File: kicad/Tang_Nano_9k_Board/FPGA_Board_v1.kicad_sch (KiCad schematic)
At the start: 51 parts, among them J1 Conn_01x24, J2 Conn_01x24, J3 Conn_01x08, J4 Conn_01x04, J5 Conn_01x04, J6 Conn_01x04, J7 Conn_01x04, Q1 PMOS, Q2 PMOS, Q3 PMOS, Q4 PMOS, Q5 PMOS, Q6 PMOS, Q7 PMOS, Q8 PMOS, SW1 SW_DIP_x08, SW2 SW_Push, SW3 SW_Push, SW4 SW_Push, U3 TBD62083AFG, U4 74HC138

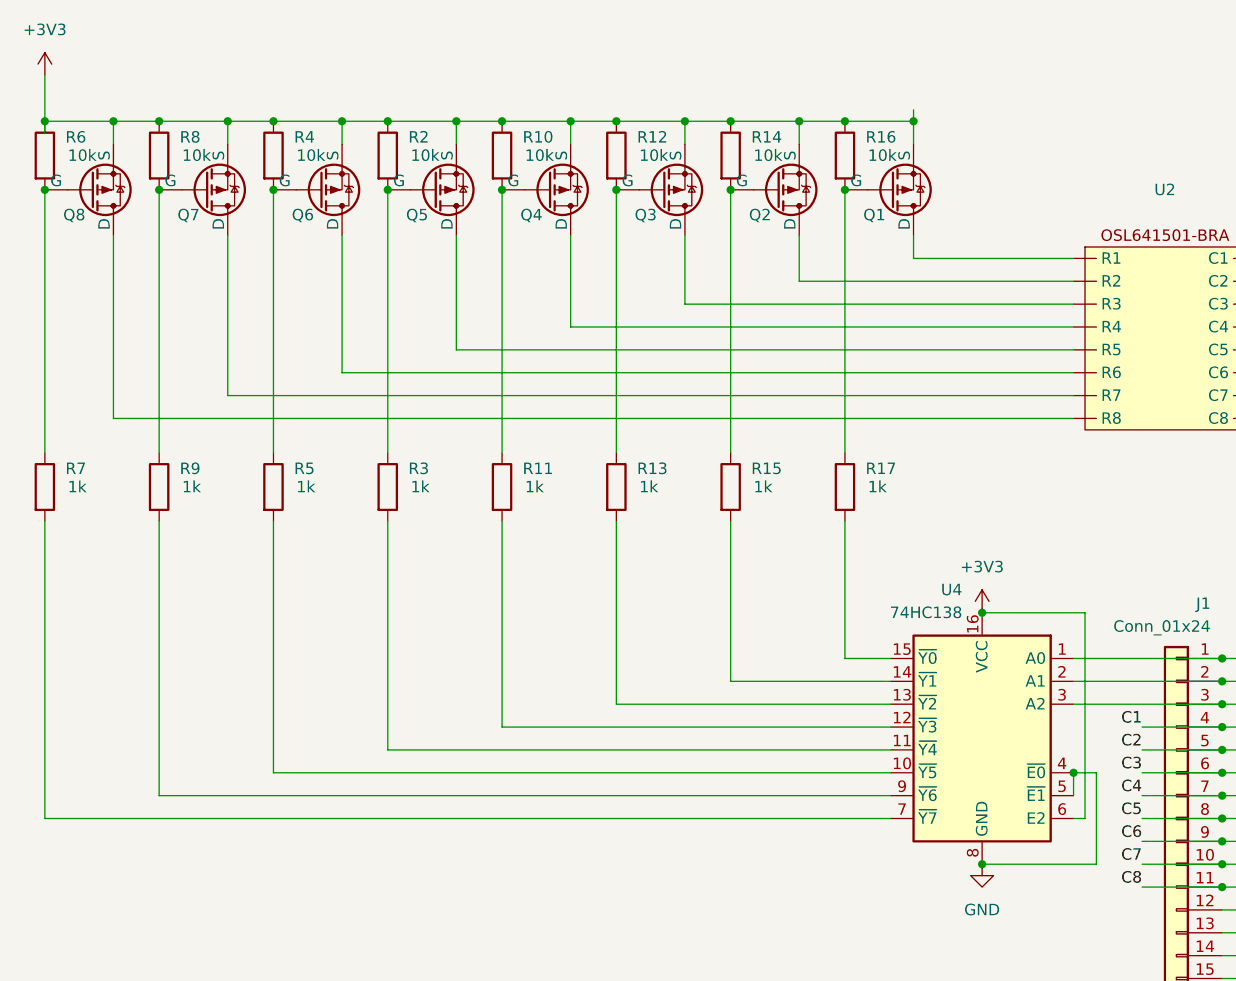
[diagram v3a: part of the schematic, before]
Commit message: set footprint
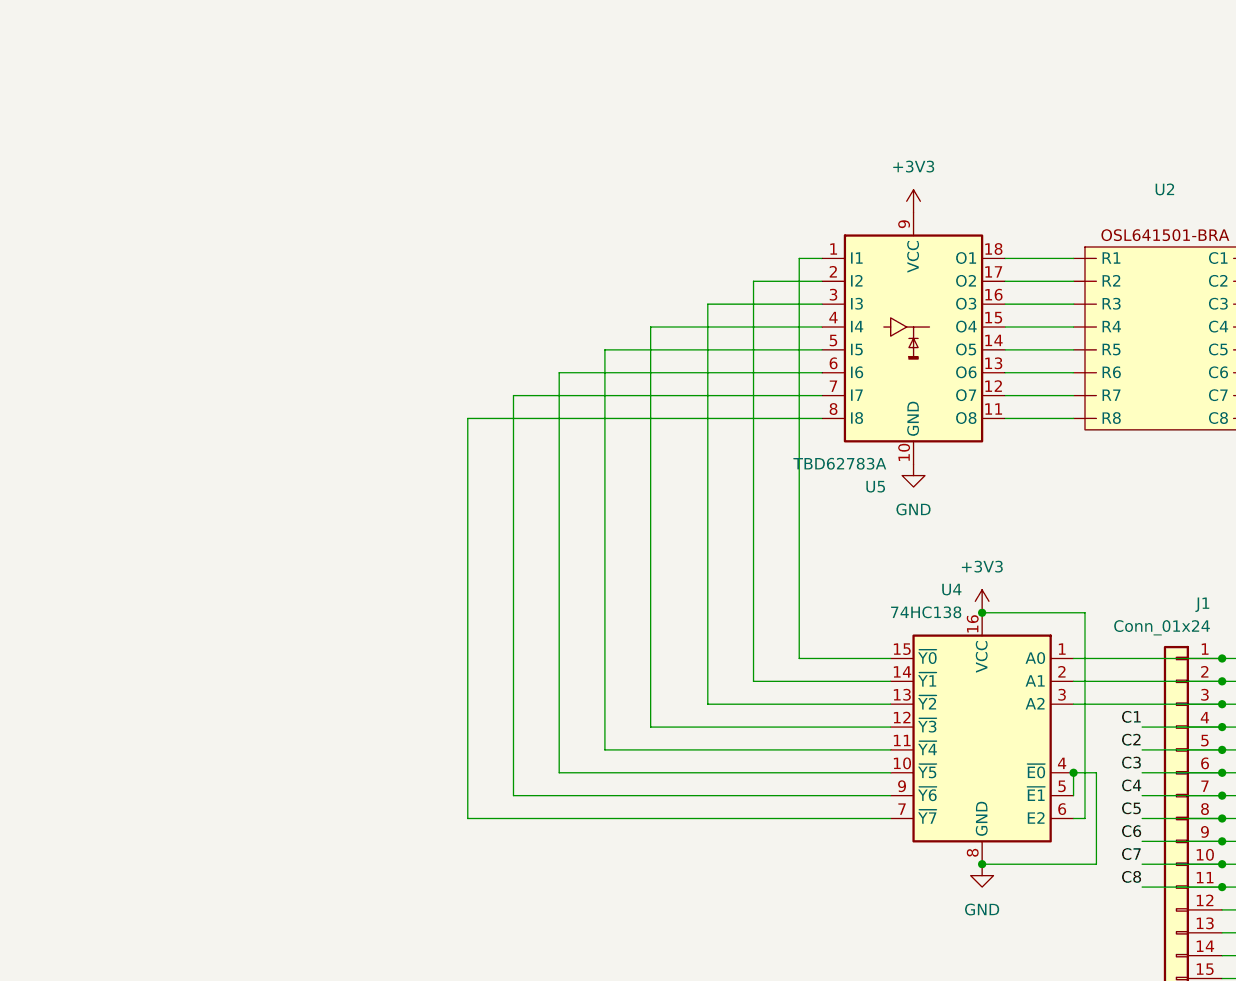
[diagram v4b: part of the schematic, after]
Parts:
- removed Q1, Q2, Q3, Q4, Q5, Q6, Q7, Q8: PMOS, symbol Simulation_SPICE:PMOS
- removed R10, R12, R14, R16, R2, R4, R6, R8: 10k, symbol Device:R
- removed R11, R13, R15, R17, R3, R5, R7, R9: 1k, symbol Device:R
- added U5: TBD62783A, Package_DIP:DIP-18_W7.62mm, symbol Transistor_Array:TBD62783A
- H1, H2, H3, H4: footprint (none) -> MountingHole:MountingHole_2.1mm
- J1, J2: footprint (none) -> Connector_PinHeader_2.54mm:PinHeader_1x24_P2.54mm_Vertical
- J3: footprint (none) -> Connector_PinHeader_2.54mm:PinHeader_1x08_P2.54mm_Vertical
- J4, J5, J6, J7: footprint (none) -> Connector_PinHeader_2.54mm:PinHeader_1x04_P2.54mm_Vertical
- R18, R19, R20, R21, R22, R23, R24, R25: footprint (none) -> Resistor_THT:R_Axial_DIN0207_L6.3mm_D2.5mm_P7.62mm_Horizontal
- SW1: footprint (none) -> Button_Switch_THT:SW_DIP_SPSTx07_Slide_9.78x19.96mm_W7.62mm_P2.54mm
- SW2, SW3, SW4: footprint (none) -> Button_Switch_SMD:Panasonic_EVQPUJ_EVQPUA
- U1: footprint (none) -> BFP:Tang_Nano_9K
- U2: footprint (none) -> BFP:OSL641501-BX
- U4: footprint (none) -> Package_DIP:CERDIP-16_W7.62mm_SideBrazed
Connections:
- net +3V3: now also U5.9 (VCC)
- net GND: now also U5.10 (GND)
- net at U2. (R8): now also U5.18 (O1)
- net at U4.13 (~{Y2}): now also U5.3 (I3)
- net at U4.14 (~{Y1}): now also U5.2 (I2)
- net at U4.10 (~{Y5}): now also U5.6 (I6)
- net at U4.11 (~{Y4}): now also U5.5 (I5)
- net at U4.12 (~{Y3}): now also U5.4 (I4)
- net at U4.15 (~{Y0}): now also U5.1 (I1)
- net at U4.7 (~{Y7}): now also U5.8 (I8)
- net at U4.9 (~{Y6}): now also U5.7 (I7)
- new net: U2. (R8), U5.11 (O8)
- new net: U2. (R8), U5.12 (O7)
- new net: U2. (R8), U5.13 (O6)
- new net: U2. (R8), U5.14 (O5)
- new net: U2. (R8), U5.15 (O4)
- new net: U2. (R8), U5.16 (O3)
- new net: U2. (R8), U5.17 (O2)

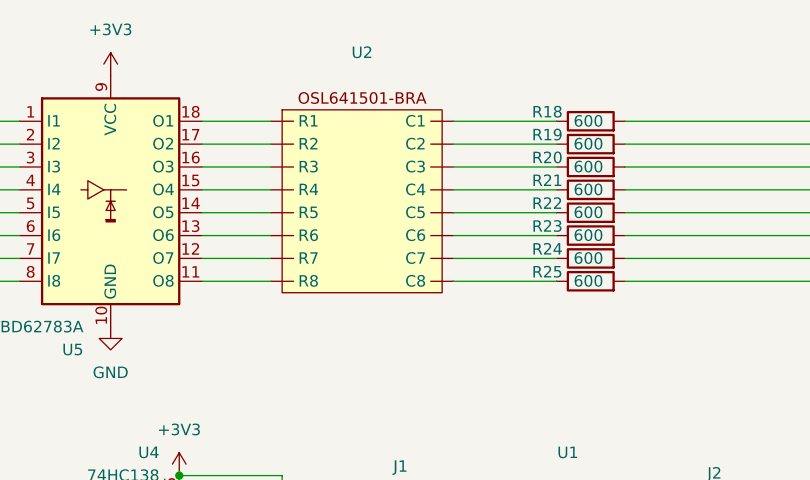
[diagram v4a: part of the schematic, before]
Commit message: making pcb board
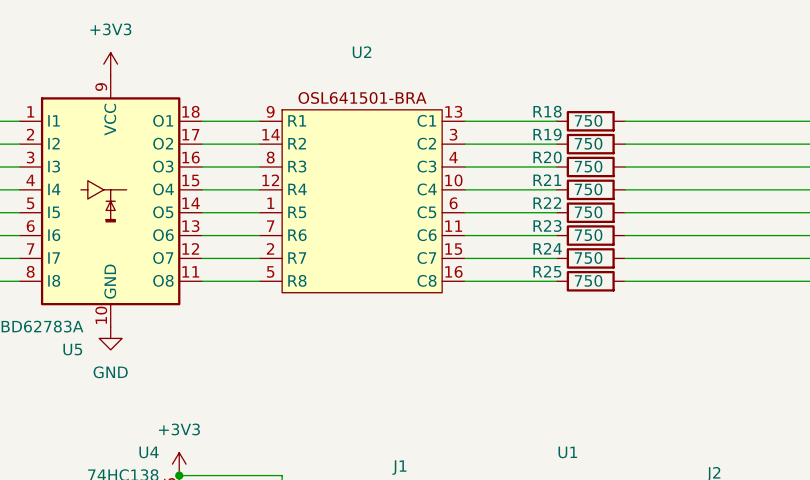
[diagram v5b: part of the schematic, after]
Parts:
- R18, R19, R20, R21, R22, R23, R24, R25: value 600 -> 750
- SW1: footprint Button_Switch_THT:SW_DIP_SPSTx07_Slide_9.78x19.96mm_W7.62mm_P2.54mm -> Button_Switch_THT:SW_DIP_SPSTx08_Slide_9.78x22.5mm_W7.62mm_P2.54mm
- U1: footprint BFP:Tang_Nano_9K -> BFP_footprints:Tang_Nano_9K
- U2: footprint BFP:OSL641501-BX -> BFP_footprints:OSL641501-BX
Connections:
- net at R19.1: now also U2.3 (C2); no longer U2. (R8)
- net at R25.1: now also U2.16 (C8); no longer U2. (R8)
- net at R18.1: now also U2.13 (C1); no longer U2. (R8)
- net at R24.1: now also U2.15 (C7); no longer U2. (R8)
- net at R21.1: now also U2.10 (C4); no longer U2. (R8)
- net at R20.1: now also U2.4 (C3); no longer U2. (R8)
- net at R23.1: now also U2.11 (C6); no longer U2. (R8)
- net at R22.1: now also U2.6 (C5); no longer U2. (R8)
- net at U5.11 (O8): now also U2.5 (R8); no longer U2. (R8)
- net at U5.12 (O7): now also U2.2 (R7); no longer U2. (R8)
- net at U5.13 (O6): now also U2.7 (R6); no longer U2. (R8)
- net at U5.14 (O5): now also U2.1 (R5); no longer U2. (R8)
- net at U5.15 (O4): now also U2.12 (R4); no longer U2. (R8)
- net at U5.16 (O3): now also U2.8 (R3); no longer U2. (R8)
- net at U5.17 (O2): now also U2.14 (R2); no longer U2. (R8)
- net at U5.18 (O1): now also U2.9 (R1); no longer U2. (R8)
